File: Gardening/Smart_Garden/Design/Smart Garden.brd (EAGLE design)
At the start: 86 x 79 mm, 77 parts, among them IC1 7809DT, IC2 LM1117-3.3, IC3 7805DT, IC4 7812DT, J1 AUDIO_JACK_TRRSSMD_RA, J2 AUDIO_JACK_TRRSSMD_RA, J3 AUDIO_JACK_TRRSSMD_RA, J4 AUDIO_JACK_TRRSSMD_RA, T1 BC847, T2 BC847, T3 BC847, T4 BC847, U1 ESP-32S, U4 MB6S

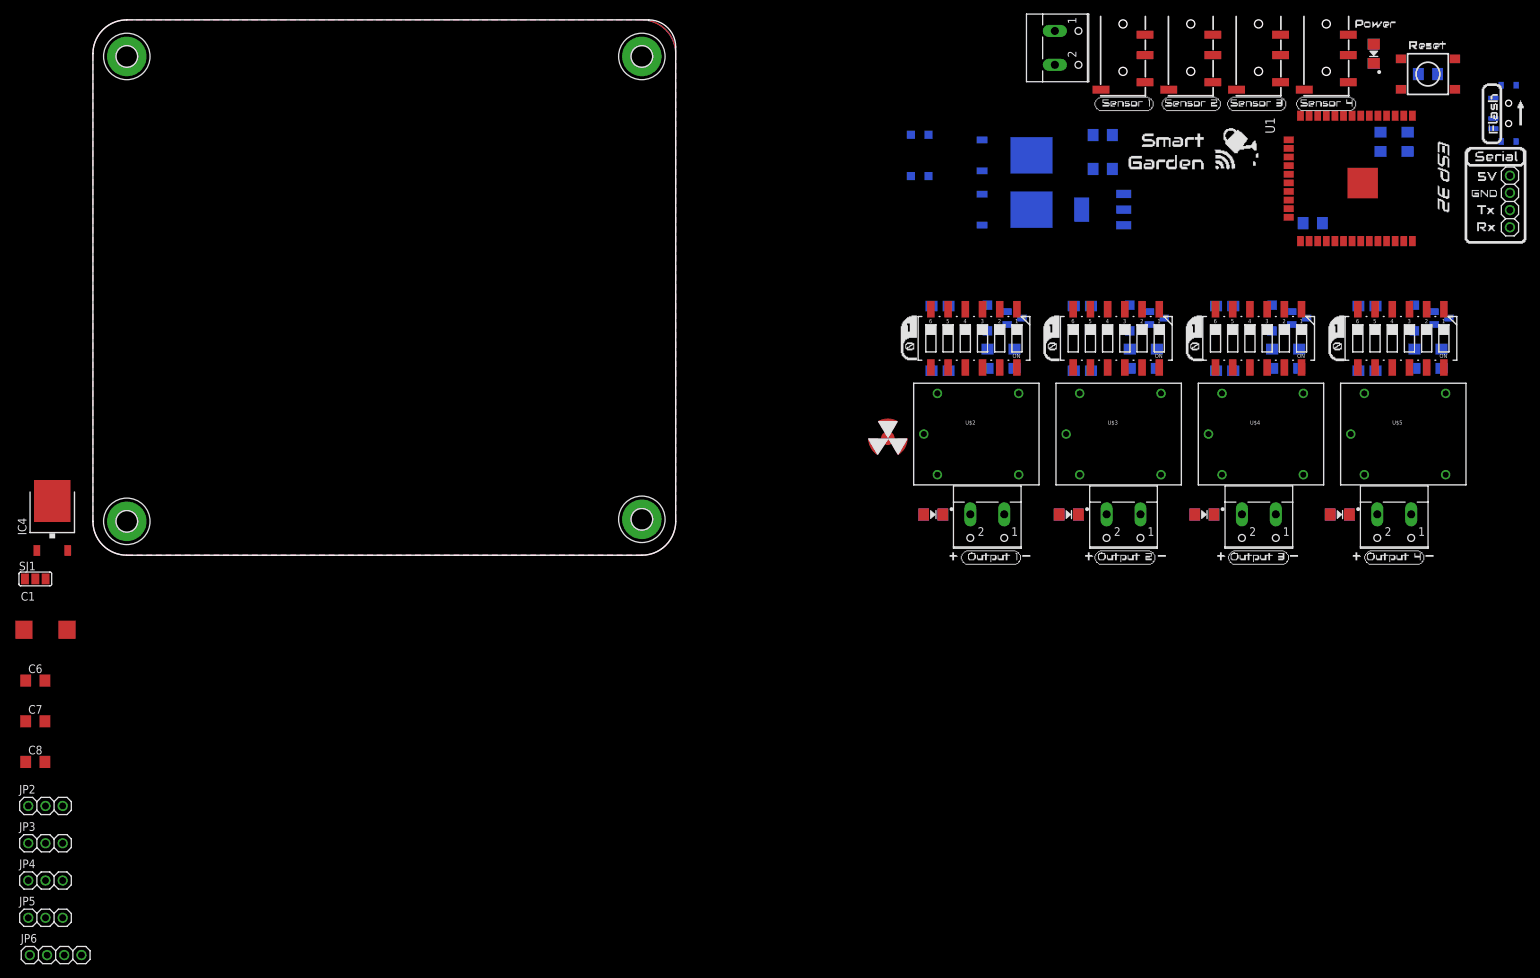
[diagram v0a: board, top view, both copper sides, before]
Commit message: Updated Design files
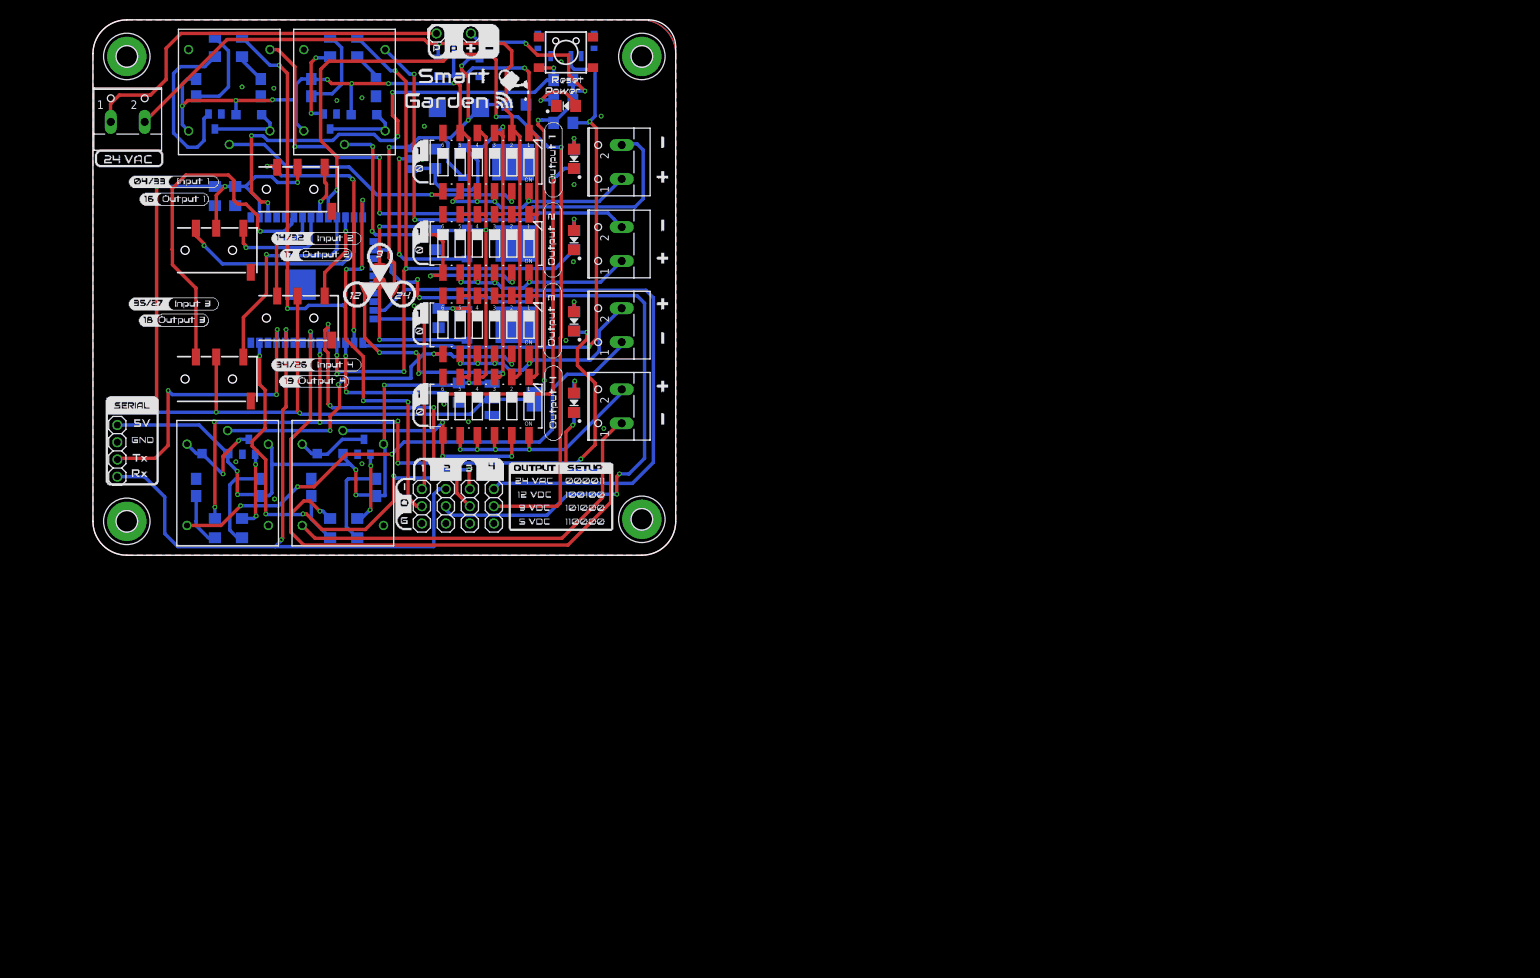
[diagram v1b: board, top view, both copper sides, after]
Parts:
- moved JP1 208.8 mm to (3.60, 15.4)
- moved J1 178.4 mm to (12.0, 26.0), turned to 0 degrees
- moved C4 173.2 mm to (21.0, 53.0), turned to 270 degrees
- moved C5 172.2 mm to (18.0, 53.0), turned to 270 degrees
- moved R10 165.9 mm to (35.0, 4.00), turned to 90 degrees
- moved R9 161.9 mm to (18.0, 4.00), turned to 90 degrees
- moved D5 161.2 mm to (35.0, 15.0), turned to 0 degrees
- moved T4 160.1 mm to (40.0, 16.0), turned to 0 degrees
- moved U1 158.1 mm to (30.3, 40.6), flipped to the bottom
- moved R6 158.0 mm to (39.0, 4.00)
- moved D4 157.3 mm to (18.0, 15.0), turned to 0 degrees
- moved T3 156.2 mm to (23.0, 16.0), turned to 0 degrees
- moved U$5 156.2 mm to (37.0, 11.0), turned to 270 degrees
- moved J2 154.7 mm to (24.0, 35.0), turned to 0 degrees
- moved R5 154.0 mm to (22.0, 4.00)
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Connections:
- removed net IO3: JP3.3
- net 1R1: now also X7.1; no longer X7.2
- net 2R1: now also X8.1; no longer X8.2
- net IO13: no longer J3.RING2
- net IO14: now also J3.RING2
- net N$1: now also X8.2; no longer X8.1
- net N$2: now also X7.2; no longer X7.1
- net RX: now also JP3.3
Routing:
- net 3V3: track 0.00 -> 230.0 mm, vias 0 -> 10
- net 5V: track 0.00 -> 214.4 mm, vias 0 -> 14
- net IO25: track 0.00 -> 132.9 mm, vias 0 -> 3
- net IO16: track 0.00 -> 131.1 mm, vias 0 -> 6
- net 24V2: track 0.00 -> 115.3 mm, vias 0 -> 1
- net IO19: track 0.00 -> 111.1 mm, vias 0 -> 5
- net IO18: track 0.00 -> 110.0 mm, vias 0 -> 8
- net IO13: track 0.00 -> 105.2 mm, vias 0 -> 4
- net 12V: track 0.00 -> 99.0 mm, vias 0 -> 5
- net RX: track 0.00 -> 98.7 mm, vias 0 -> 2
- net IO17: track 0.00 -> 93.5 mm, vias 0 -> 5
- net IO15: track 0.00 -> 93.0 mm
- net N$2: track 0.00 -> 88.5 mm, vias 0 -> 3
- net IO0: track 0.00 -> 83.6 mm, vias 0 -> 2
- net N$4: track 0.00 -> 79.1 mm, vias 0 -> 3
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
